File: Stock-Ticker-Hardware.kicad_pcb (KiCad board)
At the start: 2 copper layers, 60 x 50 mm, 19 parts, among them J1 Conn_01x05_Socket, J2 Conn_01x03_Pin, J3 Conn_01x03_Socket, J4 Conn_01x02_Pin, J5 Conn_01x02_Pin, J6 Conn_01x02_Pin, SW1 SW_Push, U1 74AHCT125

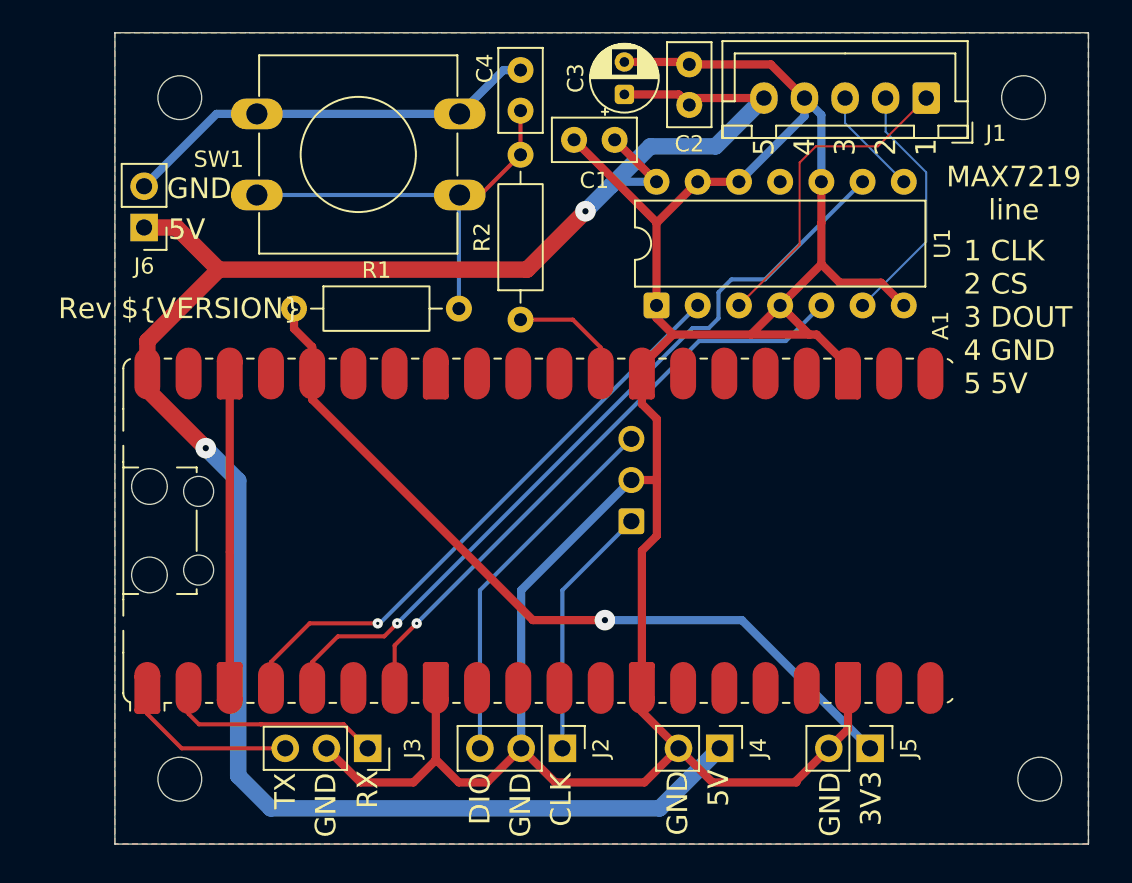
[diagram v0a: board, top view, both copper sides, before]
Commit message: Cleanup tracks
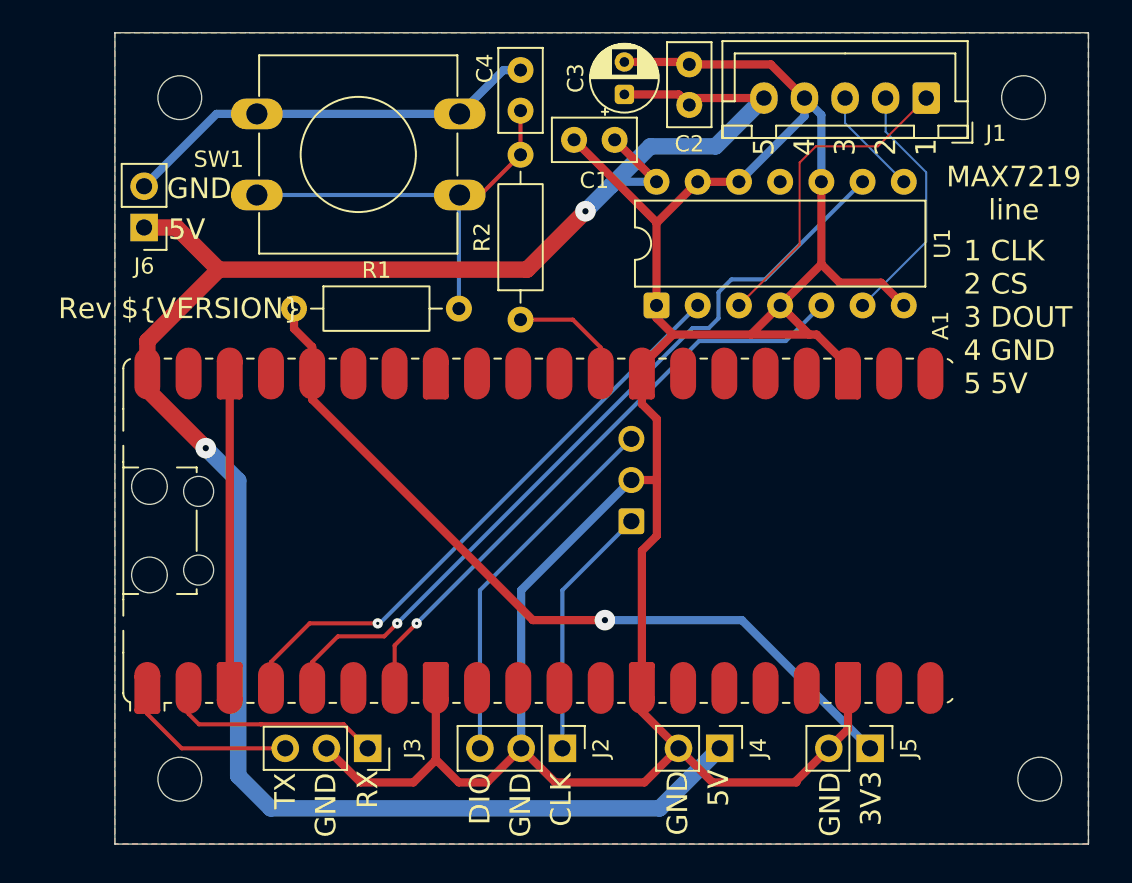
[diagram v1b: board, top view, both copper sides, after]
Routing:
- net GND: track 218.5 -> 216.4 mm
- net +5V: track 127.5 -> 125.6 mm
- net Net-(C4-Pad1): track 27.1 -> 25.7 mm
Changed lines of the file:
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@@
-	)
-	(segment
-		(start 85.25 51.8)
-		(end 85.4 51.95)
-		(width 0.508)
-		(layer "F.Cu")
-		(net 14)
-	)
-	(segment
-		(start 57.08 70.529584)
-		(end 57.08 71)
-		(width 0.508)
-		(layer "F.Cu")
-		(net 14)
 	)
 	(segment
@@
 	)
 	(segment
-		(start 93.54 61.725)
+		(start 93.54 59.185)
 		(end 93.54 64.265)
 		(width 0.508)
@@
 	)
 	(segment
-		(start 93.54 59.185)
-		(end 93.54 61.725)
-		(width 0.508)
-		(layer "F.Cu")
-		(net 14)
-	)
-	(segment
-		(start 71.25 55)
-		(end 71.7 55)
-		(width 0.508)
-		(layer "F.Cu")
-		(net 14)
-	)
-	(segment
 		(start 84.4 68.6)
 		(end 82.48 70.52)
@@
 	)
 	(segment
-		(start 91 66.805)
-		(end 91.005 66.805)
-		(width 0.508)
-		(layer "F.Cu")
-		(net 14)
-	)
-	(segment
-		(start 57.08 82)
-		(end 57.08 71)
-		(width 0.508)
-		(layer "F.Cu")
-		(net 14)
-	)
-	(segment
 		(start 94 94.1)
 		(end 95.18 92.92)
@@
 	(segment
 		(start 57.08 90.38)
-		(end 57.08 82)
+		(end 57.08 71)
 		(width 0.508)
 		(layer "F.Cu")
@@
 	)
 	(segment
-		(start 91 66.805)
-		(end 90.995 66.805)
-		(width 0.508)
-		(layer "F.Cu")
-		(net 14)
-	)
-	(segment
-		(start 82.48 70.52)
-		(end 82.48 71)
-		(width 0.508)
-		(layer "F.Cu")
-		(net 14)
-	)
-	(segment
 		(start 71.2 96.2)
 		(end 72.94 96.2)
@@
 		(start 81.4 51.8)
 		(end 85.25 51.8)
-		(width 0.508)
-		(layer "F.Cu")
-		(net 14)
-	)
-	(segment
-		(start 95.18 71)
-		(end 95.18 70.529584)
 		(width 0.508)
 		(layer "F.Cu")
@@
 	)
 	(segment
-		(start 89.575 54.45)
-		(end 90 54.025)
-		(width 0.508)
-		(layer "F.Cu")
-		(net 32)
-	)
-	(segment
 		(start 84.75 53.8)
 		(end 85.4 54.45)
@@
 	)
 	(segment
-		(start 52 71)
-		(end 52 72)
-		(width 1.016)
-		(layer "F.Cu")
-		(net 32)
-	)
-	(segment
 		(start 53.8 62)
 		(end 51.8 62)
@@
 	)
 	(segment
-		(start 83.38 59.185)
-		(end 83.38 59.18)
-		(width 0.508)
-		(layer "F.Cu")
-		(net 32)
-	)
-	(segment
 		(start 90 54.025)
 		(end 85.825 54.025)
-		(width 0.508)
-		(layer "F.Cu")
-		(net 32)
-	)
-	(segment
-		(start 83.38 59.185)
-		(end 83.065 59.185)
 		(width 0.508)
 		(layer "F.Cu")
@@
 	)
 	(segment
-		(start 71.25 66.95)
-		(end 71.2 67)
-		(width 0.254)
-		(layer "F.Cu")
-		(net 41)
-	)
-	(segment
-		(start 71.25 60)
-		(end 72.52 60)
-		(width 0.254)
-		(layer "F.Cu")
-		(net 41)
-	)
-	(segment
 		(start 75 54.8)
 		(end 75 57.52)
@@
 		(width 0.254)
 		(layer "B.Cu")
-		(net 41)
-	)
-	(segment
-		(start 71.2 60.05)
-		(end 71.25 60)
-		(width 0.254)
-		(layer "B.Cu")
